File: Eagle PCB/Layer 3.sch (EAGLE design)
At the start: 88 parts, among them Q1 AO3402, Q2 AO3402, X1 SM06B-SRSS-TB, Y1 8MHz

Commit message: Hello
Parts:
- removed 3RD_LAYER: (no value), SparkFun-Connectors:CONN_05LOCK
- removed ESC_IN, SERVO_IO: (no value), SparkFun-Connectors:CONN_03LOCK
- removed ESC_OUT: XT30PB-F, JH:XT30PB-F
- removed Q1, Q2: AO3402, SparkFun-DiscreteSemi:MOSFET-NCH-AO3404A
- removed R10, R11, R12, R13: 4.7k, JH:RESISTOR0603
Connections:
- removed net ESC_HV: ESC_IN.3, Q1.D, R10.2
- removed net N$4: ESC_IN.2
- removed net SERVO_HV: Q2.D, R12.2, SERVO_IO.3
- removed net V_BATT: ESC_OUT.P$V+
- net 3.3V: no longer 3RD_LAYER.2, Q1.G, Q2.G, R11.1, R13.1
- net 5V: no longer 3RD_LAYER.5, R10.1, R12.1, SERVO_IO.2
- net ESC_LV: no longer 3RD_LAYER.4, Q1.S, R11.2
- net GND: no longer 3RD_LAYER.1, ESC_IN.1, ESC_OUT.P$V-, SERVO_IO.1
- net SERVO_LV: no longer 3RD_LAYER.3, Q2.S, R13.2

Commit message: FUCK YOU
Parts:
- added 3RD_LAYER: (no value), SparkFun-Connectors:CONN_05LOCK
- added ESC_IN, SERVO_IO: (no value), SparkFun-Connectors:CONN_03LOCK
- added ESC_OUT: XT30PB-F, JH:XT30PB-F
- added Q1, Q2: AO3402, SparkFun-DiscreteSemi:MOSFET-NCH-AO3404A
- added R10, R11, R12, R13: 4.7k, JH:RESISTOR0603
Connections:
- new net ESC_HV: ESC_IN.3, Q1.D, R10.2
- new net N$4: ESC_IN.2
- new net SERVO_HV: Q2.D, R12.2, SERVO_IO.3
- new net V_BATT: ESC_OUT.P$V+
- net 3.3V: now also 3RD_LAYER.2, Q1.G, Q2.G, R11.1, R13.1
- net 5V: now also 3RD_LAYER.5, R10.1, R12.1, SERVO_IO.2
- net ESC_LV: now also 3RD_LAYER.4, Q1.S, R11.2
- net GND: now also 3RD_LAYER.1, ESC_IN.1, ESC_OUT.P$V-, SERVO_IO.1
- net SERVO_LV: now also 3RD_LAYER.3, Q2.S, R13.2

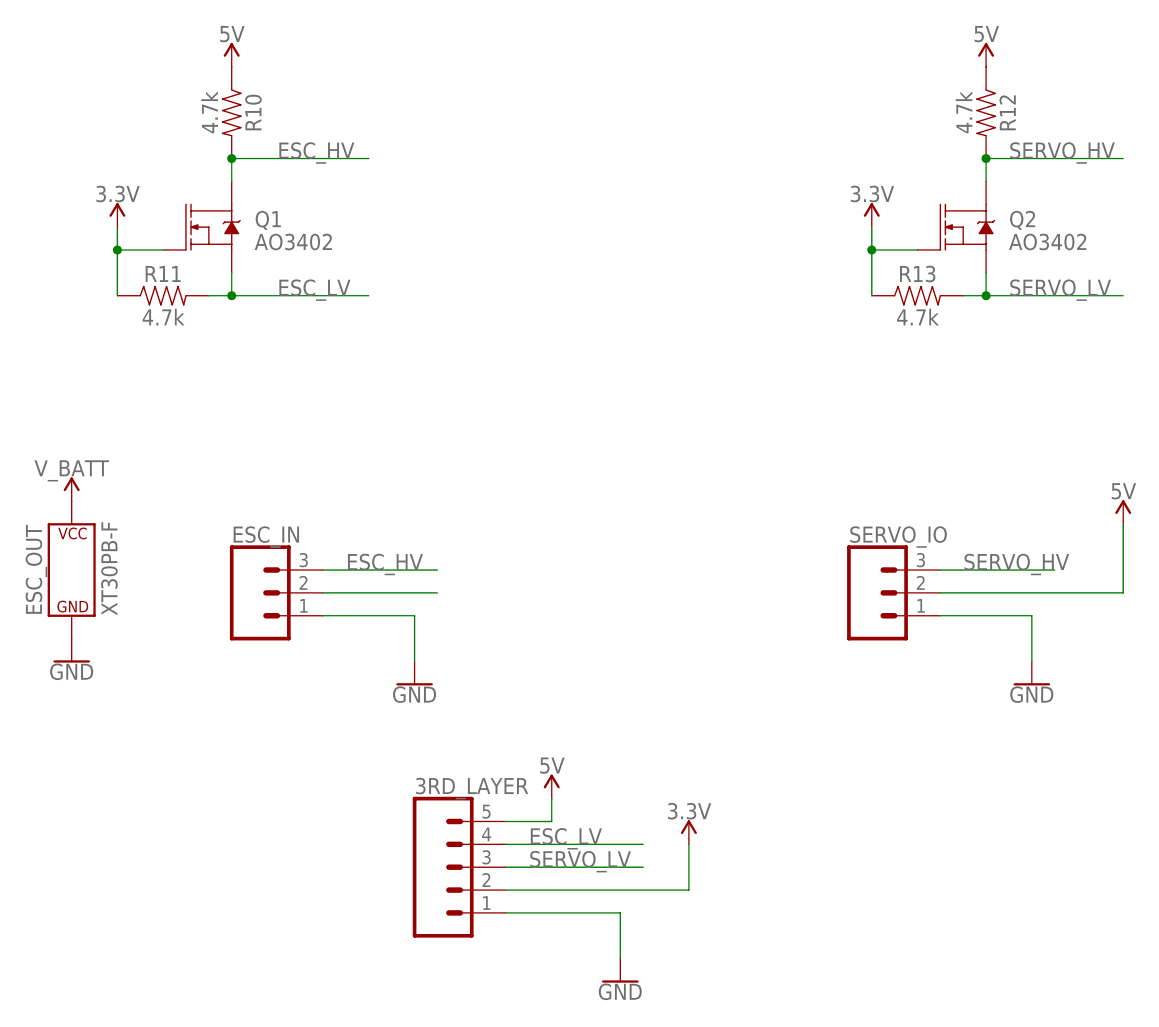
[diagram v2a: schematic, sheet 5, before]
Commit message: Done
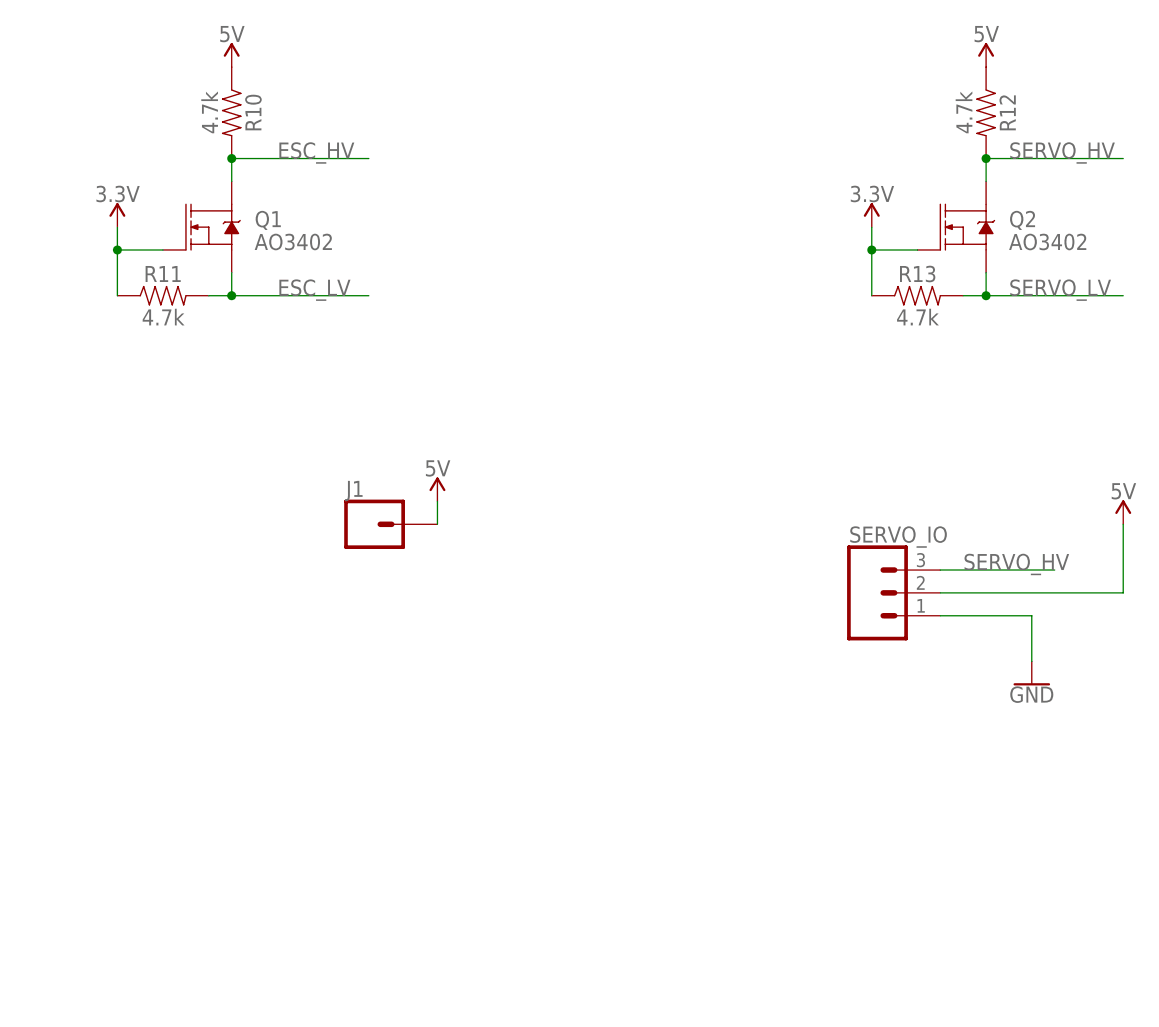
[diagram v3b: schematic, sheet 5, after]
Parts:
- removed 3RD_LAYER: (no value), SparkFun-Connectors:CONN_05LOCK
- removed ESC_IN: (no value), SparkFun-Connectors:CONN_03LOCK
- removed ESC_OUT: XT30PB-F, JH:XT30PB-F
- added J1: (no value), Connectors:CONN_01
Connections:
- removed net N$4: ESC_IN.2
- removed net V_BATT: ESC_OUT.P$V+
- net 3.3V: no longer 3RD_LAYER.2
- net 5V: now also J1.1; no longer 3RD_LAYER.5
- net ESC_HV: no longer ESC_IN.3
- net ESC_LV: no longer 3RD_LAYER.4
- net GND: no longer 3RD_LAYER.1, ESC_IN.1, ESC_OUT.P$V-
- net SERVO_LV: no longer 3RD_LAYER.3
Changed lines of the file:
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@@
 <part name="SUPPLY7" library="SparkFun-PowerSymbols" deviceset="5V" device=""/>
 <part name="SUPPLY8" library="SparkFun-PowerSymbols" deviceset="3.3V" device=""/>
-<part name="GND41" library="SparkFun-PowerSymbols" deviceset="GND" device=""/>
 <part name="GND42" library="SparkFun-PowerSymbols" deviceset="GND" device=""/>
 <part name="SUPPLY9" library="SparkFun-PowerSymbols" deviceset="5V" device=""/>
-<part name="SUPPLY3" library="SparkFun-PowerSymbols" deviceset="V_BATT" device=""/>
-<part name="GND43" library="SparkFun-PowerSymbols" deviceset="GND" device=""/>
-<part name="GND44" library="SparkFun-PowerSymbols" deviceset="GND" device=""/>
-<part name="SUPPLY10" library="SparkFun-PowerSymbols" deviceset="3.3V" device=""/>
-<part name="ESC_IN" library="SparkFun-Connectors" library_urn="urn:adsk.eagle:library:11010760" deviceset="CONN_03" device="LOCK" package3d_urn="urn:adsk.eagle:package:11011273/2"/>
 <part name="SERVO_IO" library="SparkFun-Connectors" library_urn="urn:adsk.eagle:library:11010760" deviceset="CONN_03" device="LOCK" package3d_urn="urn:adsk.eagle:package:11011273/2"/>
-<part name="ESC_OUT" library="JH" library_urn="urn:adsk.eagle:library:6027132" deviceset="XT30" device="PB-F" package3d_urn="urn:adsk.eagle:package:15925142/7"/>
-<part name="SUPPLY11" library="SparkFun-PowerSymbols" deviceset="5V" device=""/>
-<part name="3RD_LAYER" library="SparkFun-Connectors" library_urn="urn:adsk.eagle:library:11010760" deviceset="CONN_05" device="LOCK" package3d_urn="urn:adsk.eagle:package:11011302/2"/>
+<part name="J1" library="Connectors" library_urn="urn:adsk.eagle:library:19813715" deviceset="CONN_01" device="" package3d_urn="urn:adsk.eagle:package:19813825/2"/>
+<part name="SUPPLY3" library="SparkFun-PowerSymbols" deviceset="5V" device=""/>
 </parts>
 <sheets>
@@
 <attribute name="VALUE" x="149.86" y="124.714" size="1.778" layer="96" align="bottom-center"/>
 </instance>
-<instance part="GND41" gate="1" x="99.06" y="71.12" smashed="yes">
-<attribute name="VALUE" x="99.06" y="70.866" size="1.778" layer="96" align="top-center"/>
-</instance>
 <instance part="GND42" gate="1" x="167.64" y="71.12" smashed="yes">
 <attribute name="VALUE" x="167.64" y="70.866" size="1.778" layer="96" align="top-center"/>
@@
 <instance part="SUPPLY9" gate="G$1" x="177.8" y="88.9" smashed="yes">
 <attribute name="VALUE" x="177.8" y="91.694" size="1.778" layer="96" align="bottom-center"/>
-</instance>
-<instance part="SUPPLY3" gate="G$1" x="60.96" y="91.44" smashed="yes">
-<attribute name="VALUE" x="60.96" y="94.234" size="1.778" layer="96" align="bottom-center"/>
-</instance>
-<instance part="GND43" gate="1" x="60.96" y="73.66" smashed="yes">
-<attribute name="VALUE" x="60.96" y="73.406" size="1.778" layer="96" align="top-center"/>
-</instance>
-<instance part="GND44" gate="1" x="121.92" y="38.1" smashed="yes">
-<attribute name="VALUE" x="121.92" y="37.846" size="1.778" layer="96" align="top-center"/>
-</instance>
-<instance part="SUPPLY10" gate="G$1" x="129.54" y="53.34" smashed="yes">
-<attribute name="VALUE" x="129.54" y="56.134" size="1.778" layer="96" align="bottom-center"/>
-</instance>
-<instance part="ESC_IN" gate="J$1" x="81.28" y="81.28" smashed="yes">
-<attribute name="VALUE" x="78.74" y="73.914" size="1.778" layer="96" font="vector"/>
-<attribute name="NAME" x="78.74" y="86.868" size="1.778" layer="95" font="vector"/>
 </instance>
 <instance part="SERVO_IO" gate="J$1" x="149.86" y="81.28" smashed="yes">
@@
 <attribute name="NAME" x="147.32" y="86.868" size="1.778" layer="95" font="vector"/>
 </instance>
-<instance part="ESC_OUT" gate="G$1" x="60.96" y="83.82" smashed="yes">
-<attribute name="NAME" x="57.658" y="78.74" size="1.778" layer="95" font="vector" rot="R90"/>
-<attribute name="VALUE" x="66.04" y="78.74" size="1.778" layer="95" font="vector" rot="R90"/>
-</instance>
-<instance part="SUPPLY11" gate="G$1" x="114.3" y="58.42" smashed="yes">
-<attribute name="VALUE" x="114.3" y="61.214" size="1.778" layer="96" align="bottom-center"/>
-</instance>
-<instance part="3RD_LAYER" gate="G$1" x="101.6" y="50.8" smashed="yes">
-<attribute name="VALUE" x="99.06" y="40.894" size="1.778" layer="96" font="vector"/>
-<attribute name="NAME" x="99.06" y="58.928" size="1.778" layer="95" font="vector"/>
+<instance part="J1" gate="G$1" x="93.98" y="88.9" smashed="yes">
+<attribute name="VALUE" x="91.44" y="84.074" size="1.778" layer="96" font="vector"/>
+<attribute name="NAME" x="91.44" y="91.948" size="1.778" layer="95" font="vector"/>
+</instance>
+<instance part="SUPPLY3" gate="G$1" x="101.6" y="91.44" smashed="yes">
+<attribute name="VALUE" x="101.6" y="94.234" size="1.778" layer="96" align="bottom-center"/>
 </instance>
 </instances>
@@
 <label x="83.82" y="129.54" size="1.778" layer="95"/>
 </segment>
-<segment>
-<wire x1="88.9" y1="83.82" x2="101.6" y2="83.82" width="0.1524" layer="91"/>
-<label x="91.44" y="83.82" size="1.778" layer="95"/>
-<pinref part="ESC_IN" gate="J$1" pin="3"/>
-</segment>
 </net>
 <net name="5V" class="0">
@@
 </segment>
 <segment>
-<wire x1="109.22" y1="55.88" x2="114.3" y2="55.88" width="0.1524" layer="91"/>
-<wire x1="114.3" y1="55.88" x2="114.3" y2="58.42" width="0.1524" layer="91"/>
-<pinref part="SUPPLY11" gate="G$1" pin="5V"/>
-<pinref part="3RD_LAYER" gate="G$1" pin="5"/>
+<pinref part="SUPPLY3" gate="G$1" pin="5V"/>
+<pinref part="J1" gate="G$1" pin="1"/>
+<wire x1="101.6" y1="91.44" x2="101.6" y2="88.9" width="0.1524" layer="91"/>
 </segment>
 </net>
@@
 <junction x="149.86" y="119.38"/>
 </segment>
-<segment>
-<wire x1="109.22" y1="48.26" x2="129.54" y2="48.26" width="0.1524" layer="91"/>
-<wire x1="129.54" y1="48.26" x2="129.54" y2="53.34" width="0.1524" layer="91"/>
-<pinref part="SUPPLY10" gate="G$1" pin="3.3V"/>
-<pinref part="3RD_LAYER" gate="G$1" pin="2"/>
-</segment>
 </net>
 <net name="ESC_LV" class="0">
@@
 <label x="83.82" y="114.3" size="1.778" layer="95"/>
 </segment>
-<segment>
-<wire x1="109.22" y1="53.34" x2="124.46" y2="53.34" width="0.1524" layer="91"/>
-<label x="111.76" y="53.34" size="1.778" layer="95"/>
-<pinref part="3RD_LAYER" gate="G$1" pin="4"/>
-</segment>
 </net>
 <net name="SERVO_HV" class="0">
@@
 <label x="165.1" y="114.3" size="1.778" layer="95"/>
 </segment>
-<segment>
-<wire x1="109.22" y1="50.8" x2="124.46" y2="50.8" width="0.1524" layer="91"/>
-<label x="111.76" y="50.8" size="1.778" layer="95"/>
-<pinref part="3RD_LAYER" gate="G$1" pin="3"/>
-</segment>
 </net>
 <net name="GND" class="0">
-<segment>
-<wire x1="88.9" y1="78.74" x2="99.06" y2="78.74" width="0.1524" layer="91"/>
-<wire x1="99.06" y1="78.74" x2="99.06" y2="73.66" width="0.1524" layer="91"/>
-<pinref part="GND41" gate="1" pin="GND"/>
-<pinref part="ESC_IN" gate="J$1" pin="1"/>
-</segment>
 <segment>
 <wire x1="157.48" y1="78.74" x2="167.64" y2="78.74" width="0.1524" layer="91"/>
@@
 <pinref part="SERVO_IO" gate="J$1" pin="1"/>
 </segment>
-<segment>
-<wire x1="109.22" y1="45.72" x2="121.92" y2="45.72" width="0.1524" layer="91"/>
-<wire x1="121.92" y1="45.72" x2="121.92" y2="40.64" width="0.1524" layer="91"/>
-<pinref part="GND44" gate="1" pin="GND"/>
-<pinref part="3RD_LAYER" gate="G$1" pin="1"/>
-</segment>
-<segment>
-<pinref part="GND43" gate="1" pin="GND"/>
-<pinref part="ESC_OUT" gate="G$1" pin="P$V-"/>
-</segment>
-</net>
-<net name="N$4" class="0">
-<segment>
-<wire x1="88.9" y1="81.28" x2="101.6" y2="81.28" width="0.1524" layer="91"/>
-<pinref part="ESC_IN" gate="J$1" pin="2"/>
-</segment>
-</net>
-<net name="V_BATT" class="0">
-<segment>
-<pinref part="SUPPLY3" gate="G$1" pin="V_BATT"/>
-<pinref part="ESC_OUT" gate="G$1" pin="P$V+"/>
-</segment>
-</net>
+</net>
